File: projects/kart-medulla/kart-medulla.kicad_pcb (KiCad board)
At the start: 2 copper layers, 59 parts, among them CN1 1990012, CN10 1990012, CN2 1990012, CN3 1990012, CN4 1990012, CN5 1990012, CN6 1990012, CN7 1990012, CN8 1990012, CN9 1990012, Q3 IRLZ44NPBF, Q4 BSS123_C5184436, U1 LM358DR, U13 MCP4922-E/SL, U14 MAX4660EUA+T, U19 L7805CDT_C20611927, U23 SSW-122-01-T-D, U24 SSW-122-01-T-S, U25 PCF8574T/3,518, U5 SN74LVC3G17DCTR

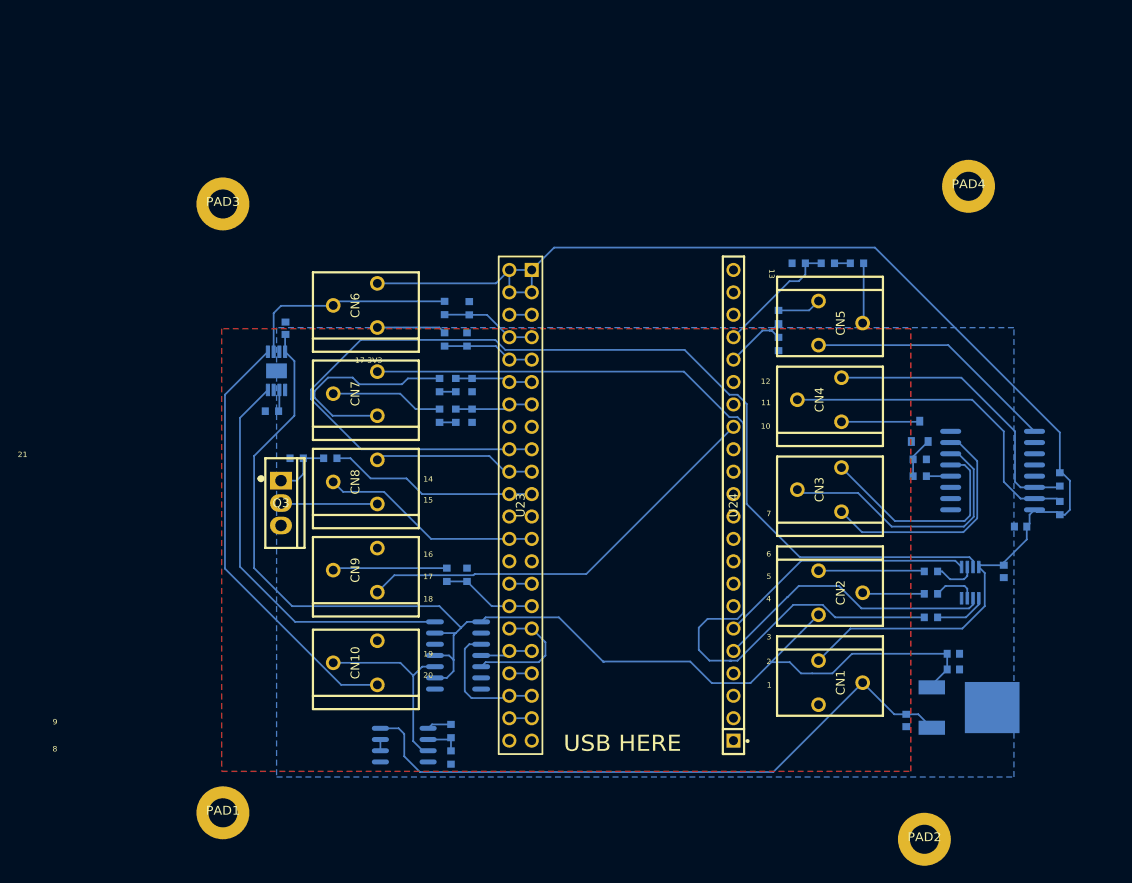
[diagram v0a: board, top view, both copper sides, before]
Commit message: refilled update
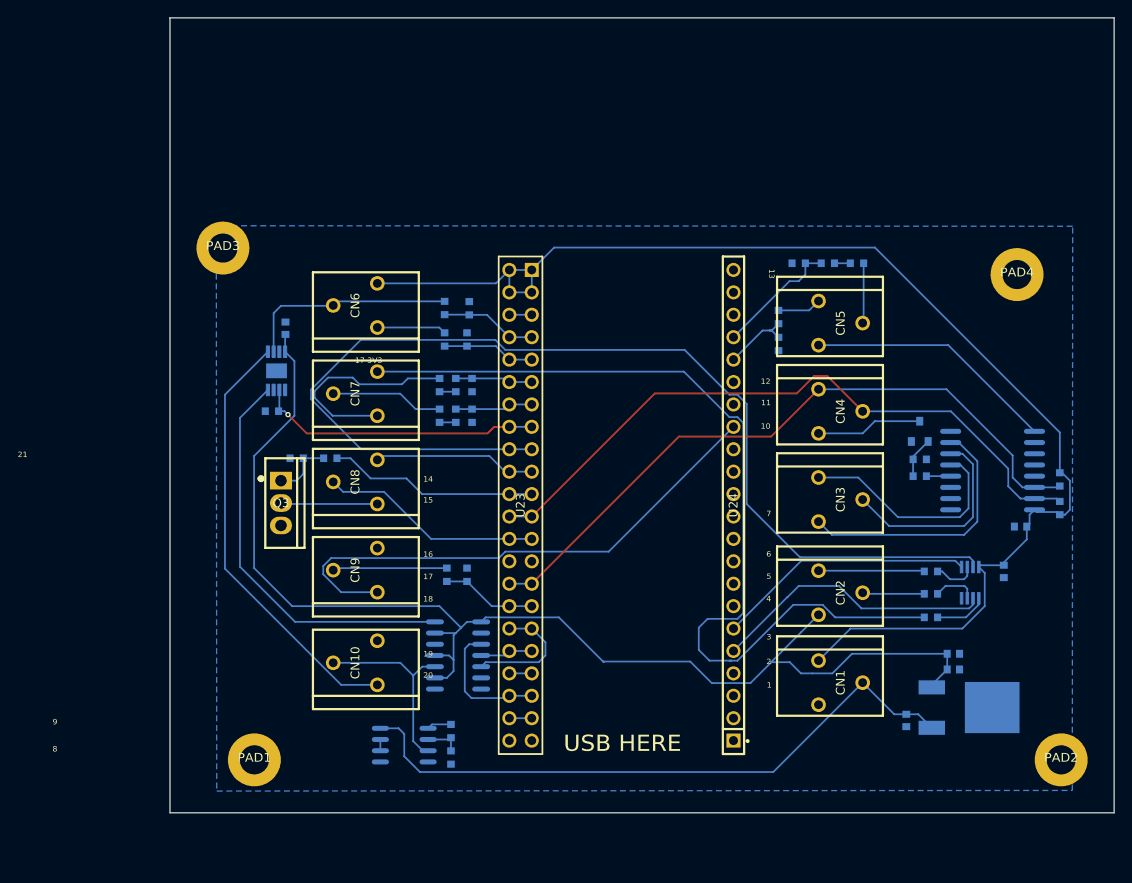
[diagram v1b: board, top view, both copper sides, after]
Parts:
- moved PAD2 17.9 mm to (157.0, 102.0)
- moved PAD4 11.4 mm to (152.0, 47.0)
- moved PAD1 6.98 mm to (65.6, 102.0)
- moved PAD3 5.00 mm to (62.0, 44.0)
- moved CN4 2.74 mm to (132.0, 62.5), turned to -90 degrees
- moved CN3 2.65 mm to (132.0, 72.5), turned to -90 degrees
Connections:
- CN3 pad 1: /P1/EXP_P3 -> /P1/EXP_P1
- CN3 pad 3: /P1/EXP_P1 -> /P1/EXP_P3
- CN4 pad 1: /P1/REVERSE_WIRE -> /P1/SCL__I2C
- CN4 pad 3: /P1/SCL__I2C -> /P1/REVERSE_WIRE
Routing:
- net /P1/SCL__I2C: track 35.8 -> 77.6 mm
- net /P1/SDA__I2C: track 37.9 -> 76.0 mm
- net /P1/SELECT_THROTTLE: track 2.44 -> 32.5 mm, vias 0 -> 1
- net /P1/CMD_STEER__PWM_3V3: track 48.1 -> 60.9 mm
- net /P1/EXP_P2: track 30.9 -> 23.2 mm
- net /P1/REVERSE_WIRE: track 8.90 -> 12.0 mm
- net /P1/EXP_P3: track 27.4 -> 30.0 mm
- net /P1/EXP_P1: track 24.9 -> 25.7 mm
- removed copper zone on F.Cu, net GND
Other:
- board outline added: 107 x 90.1 mm
